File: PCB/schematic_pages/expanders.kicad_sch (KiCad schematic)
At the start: 32 parts

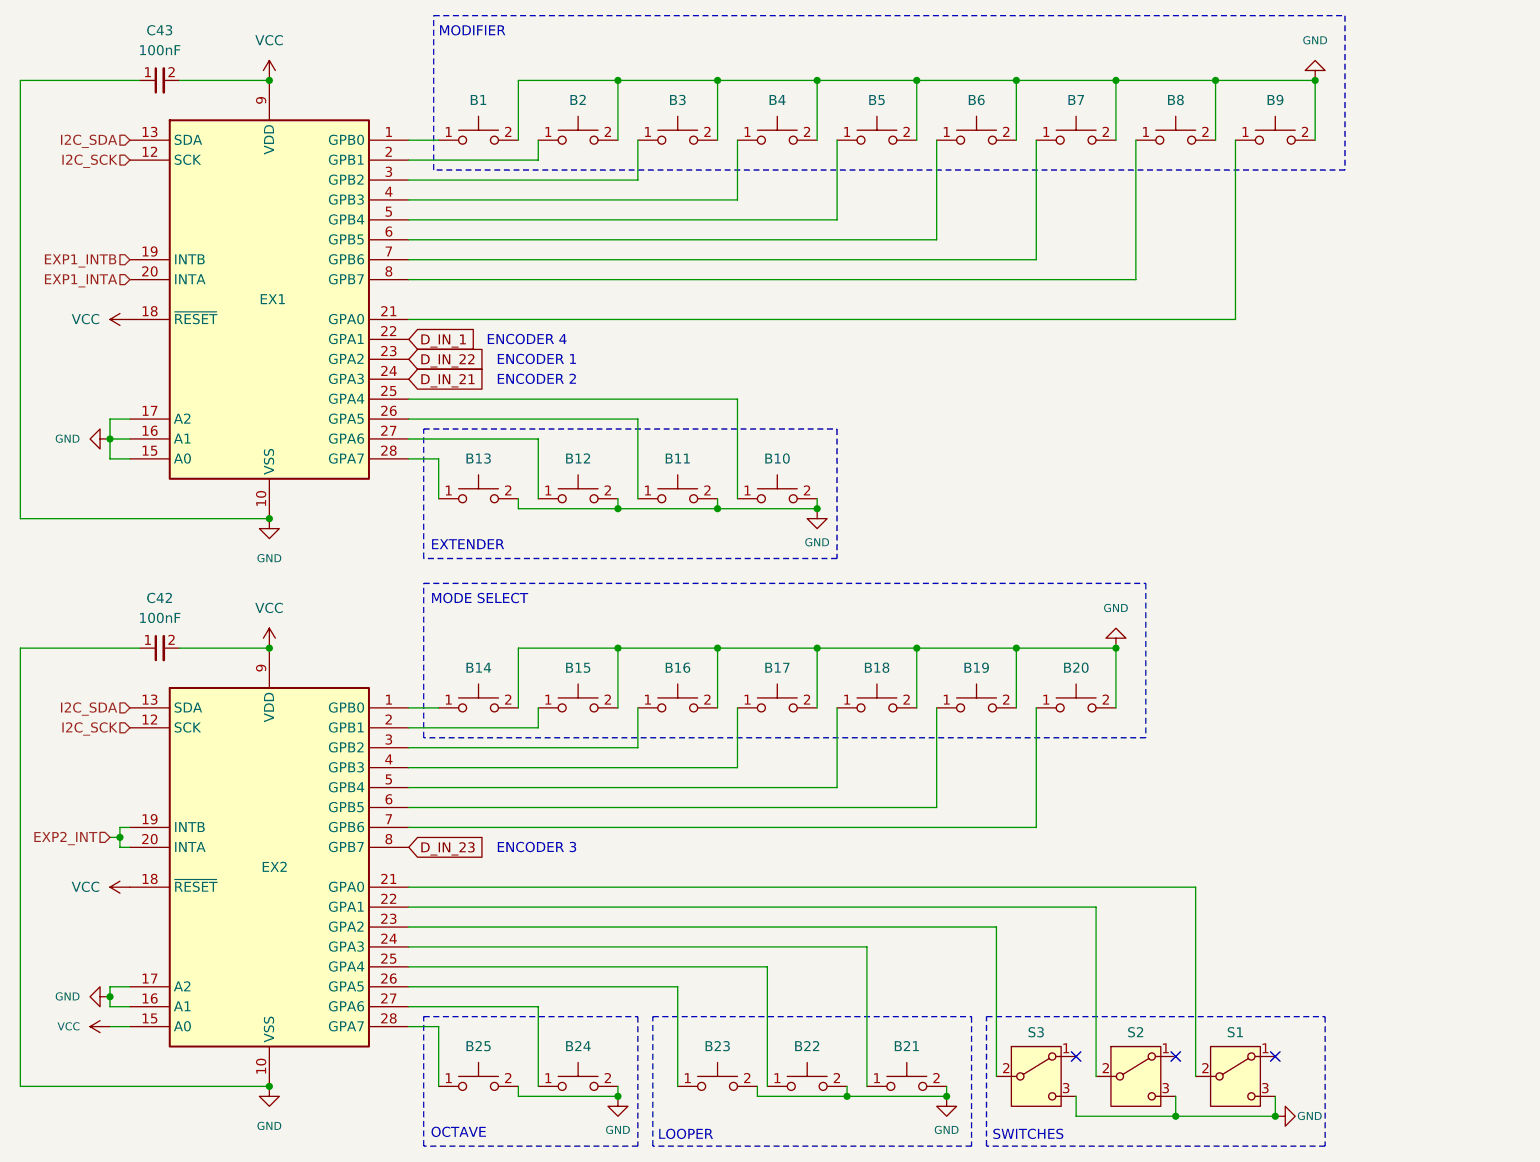
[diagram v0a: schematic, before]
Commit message: longahh day
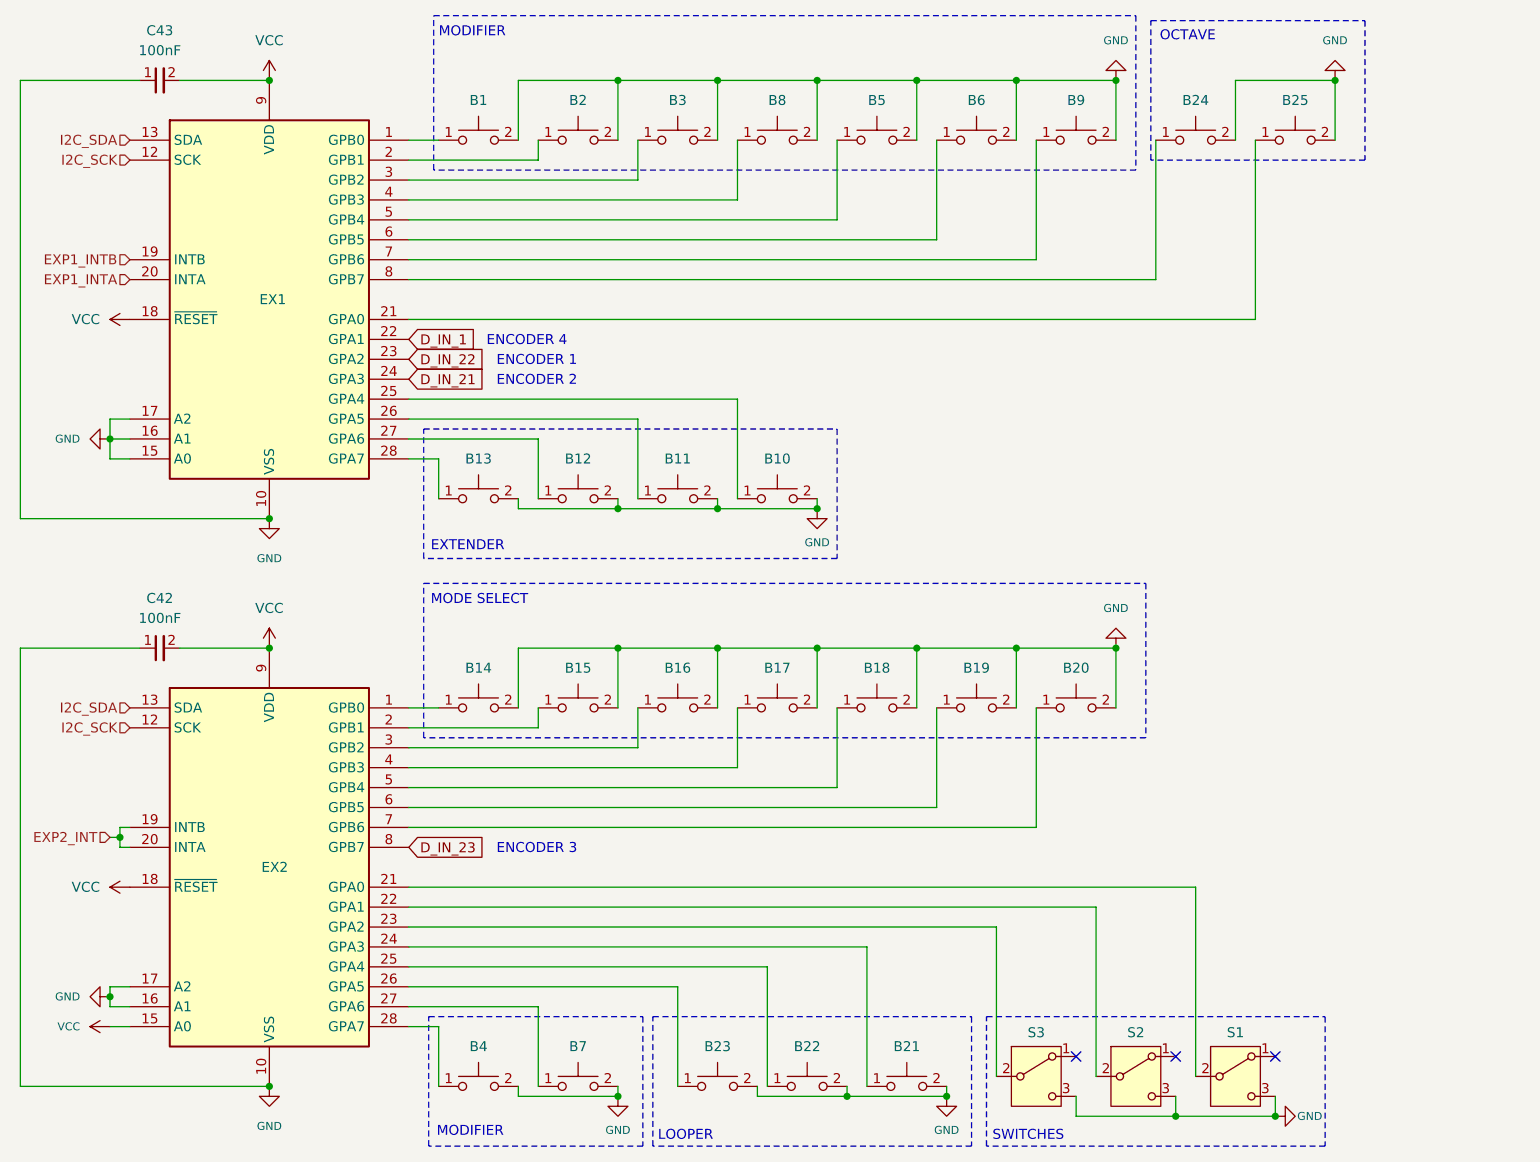
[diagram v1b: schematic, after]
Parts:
- renumbered B8 to B24, B9 to B25, B25 to B4, B24 to B7, B4 to B8, B7 to B9
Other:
- moved on the sheet: B24, B25
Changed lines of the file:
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@@
 	(paper "A4")
 	(rectangle
+		(start 105.41 143.51)
+		(end 132.715 160.02)
+		(stroke
+			(width 0)
+			(type dash)
+		)
+		(fill
+			(type none)
+		)
+	)
+	(rectangle
 		(start 176.53 143.51)
 		(end 219.71 160.02)
@@
 	(rectangle
 		(start 106.045 15.875)
-		(end 222.25 35.56)
+		(end 195.58 35.56)
 		(stroke
 			(width 0)
@@
 	)
 	(rectangle
-		(start 104.775 143.51)
-		(end 132.08 160.02)
+		(start 197.485 16.51)
+		(end 224.79 34.29)
 		(stroke
 			(width 0)
@@
 		)
 	)
+	(text "MODIFIER"
+		(exclude_from_sim no)
+		(at 106.426 158.242 0)
+		(effects
+			(font
+				(size 1.27 1.27)
+			)
+			(justify left)
+		)
+	)
 	(text "MODE SELECT"
 		(exclude_from_sim no)
@@
 	(text "OCTAVE"
 		(exclude_from_sim no)
-		(at 105.664 158.496 0)
+		(at 198.628 18.542 0)
 		(effects
 			(font
@@
 	)
 	(junction
+		(at 193.04 24.13)
+		(diameter 0)
+		(color 0 0 0 1)
+	)
+	(junction
 		(at 180.34 96.52)
 		(diameter 0)
@@
 	)
 	(junction
-		(at 218.44 24.13)
-		(diameter 0)
-		(color 0 0 0 1)
-	)
-	(junction
-		(at 193.04 24.13)
+		(at 220.98 24.13)
 		(diameter 0)
 		(color 0 0 0 1)
@@
 	)
 	(junction
-		(at 205.74 24.13)
-		(diameter 0)
-		(color 0 0 0 1)
-	)
-	(junction
 		(at 180.34 24.13)
 		(diameter 0)
@@
 	(wire
 		(pts
-			(xy 102.87 49.53) (xy 195.58 49.53)
+			(xy 102.87 49.53) (xy 198.12 49.53)
 		)
 		(stroke
@@
 	(wire
 		(pts
-			(xy 208.28 54.61) (xy 208.28 31.75)
+			(xy 210.82 54.61) (xy 210.82 31.75)
 		)
 		(stroke
@@
 	(wire
 		(pts
-			(xy 205.74 24.13) (xy 205.74 31.75)
+			(xy 208.28 24.13) (xy 208.28 31.75)
 		)
 		(stroke
@@
 	(wire
 		(pts
-			(xy 218.44 24.13) (xy 218.44 31.75)
+			(xy 220.98 24.13) (xy 220.98 31.75)
 		)
 		(stroke
@@
 	(wire
 		(pts
-			(xy 195.58 49.53) (xy 195.58 31.75)
+			(xy 198.12 49.53) (xy 198.12 31.75)
 		)
 		(stroke
@@
 	(wire
 		(pts
-			(xy 205.74 24.13) (xy 218.44 24.13)
+			(xy 208.28 24.13) (xy 220.98 24.13)
 		)
 		(stroke
@@
 	(wire
 		(pts
-			(xy 102.87 54.61) (xy 208.28 54.61)
+			(xy 102.87 54.61) (xy 210.82 54.61)
 		)
 		(stroke
@@
 	(wire
 		(pts
-			(xy 193.04 24.13) (xy 205.74 24.13)
-		)
-		(stroke
-			(width 0)
-			(type default)
-			(color 0 0 0 1)
-		)
-	)
-	(wire
-		(pts
 			(xy 102.87 36.83) (xy 132.08 36.83)
 		)
@@
 	(symbol
 		(lib_id "Symbols:GND")
-		(at 218.44 24.13 180)
+		(at 220.98 24.13 180)
 		(unit 1)
 		(exclude_from_sim no)
@@
 		(fields_autoplaced yes)
 		(property "Reference" "#PWR0106"
-			(at 218.44 24.13 0)
+			(at 220.98 24.13 0)
 			(effects
 				(font
@@
 		)
 		(property "Value" "GND"
-			(at 218.44 19.05 0)
+			(at 220.98 19.05 0)
 			(effects
 				(font
@@
 		)
 		(property "Footprint" ""
-			(at 218.44 24.13 0)
+			(at 220.98 24.13 0)
 			(effects
 				(font
@@
 		)
 		(property "Datasheet" ""
-			(at 218.44 24.13 0)
+			(at 220.98 24.13 0)
 			(effects
 				(font
@@
 		)
 		(property "Description" ""
-			(at 218.44 24.13 0)
+			(at 220.98 24.13 0)
 			(effects
 				(font
@@
 	)
 	(symbol
+		(lib_id "Symbols:GND")
+		(at 193.04 24.13 180)
+		(unit 1)
+		(exclude_from_sim no)
+		(in_bom yes)
+		(on_board yes)
+		(dnp no)
+		(fields_autoplaced yes)
+		(property "Reference" "#PWR0107"
+			(at 193.04 24.13 0)
+			(effects
+				(font
+					(size 1.27 1.27)
+				)
+				(hide yes)
+			)
+		)
+		(property "Value" "GND"
+			(at 193.04 19.05 0)
+			(effects
+				(font
+					(size 1.016 1.016)
+				)
+			)
+		)
+		(property "Footprint" ""
+			(at 193.04 24.13 0)
+			(effects
+				(font
+					(size 1.27 1.27)
+				)
+				(hide yes)
+			)
+		)
+		(property "Datasheet" ""
+			(at 193.04 24.13 0)
+			(effects
+				(font
+					(size 1.27 1.27)
+				)
+				(hide yes)
+			)
+		)
+		(property "Description" ""
+			(at 193.04 24.13 0)
+			(effects
+				(font
+					(size 1.27 1.27)
+				)
+				(hide yes)
+			)
+		)
+		(pin ""
+		)
+		(instances
+			(project "Harmora"
+				(path "/de43e009-b04c-42c1-b131-cdc664039a0d/8f5845f6-f6f8-4f8f-ac6e-d033b6efee1b"
+					(reference "#PWR0107")
+					(unit 1)
+				)
+			)
+		)
+	)
+	(symbol
 		(lib_id "power:VCC")
 		(at 67.31 127 90)
@@
 		(dnp no)
 		(fields_autoplaced yes)
-		(property "Reference" "B25"
+		(property "Reference" "B4"
 			(at 111.76 147.32 0)
 			(effects
@@
 			(project "Harmora"
 				(path "/de43e009-b04c-42c1-b131-cdc664039a0d/8f5845f6-f6f8-4f8f-ac6e-d033b6efee1b"
-					(reference "B25")
+					(reference "B4")
 					(unit 1)
 				)
@@
 		(dnp no)
 		(fields_autoplaced yes)
-		(property "Reference" "B7"
+		(property "Reference" "B9"
 			(at 187.96 26.67 0)
 			(effects
@@
 			(project "MCU_328p"
 				(path "/de43e009-b04c-42c1-b131-cdc664039a0d/8f5845f6-f6f8-4f8f-ac6e-d033b6efee1b"
-					(reference "B7")
+					(reference "B9")
 					(unit 1)
 				)
@@
 	(symbol
 		(lib_id "Symbols:Push_Switch")
-		(at 213.36 31.75 0)
+		(at 215.9 31.75 0)
 		(unit 1)
 		(exclude_from_sim no)
@@
 		(dnp no)
 		(fields_autoplaced yes)
-		(property "Reference" "B9"
-			(at 213.36 26.67 0)
+		(property "Reference" "B25"
+			(at 215.9 26.67 0)
 			(effects
 				(font
@@
 		)
 		(property "Value" "~"
-			(at 213.36 31.75 0)
+			(at 215.9 31.75 0)
 			(effects
 				(font
@@
 		)
 		(property "Footprint" "Footprints:Mechanical Switch"
-			(at 213.36 31.75 0)
+			(at 215.9 31.75 0)
 			(effects
 				(font
@@
 		)
 		(property "Datasheet" ""
-			(at 213.36 31.75 0)
+			(at 215.9 31.75 0)
 			(effects
 				(font
@@
 		)
 		(property "Description" ""
-			(at 213.36 31.75 0)
+			(at 215.9 31.75 0)
 			(effects
 				(font
@@
 			(project "MCU_328p"
 				(path "/de43e009-b04c-42c1-b131-cdc664039a0d/8f5845f6-f6f8-4f8f-ac6e-d033b6efee1b"
-					(reference "B9")
+					(reference "B25")
 					(unit 1)
 				)
@@
 		(dnp no)
 		(fields_autoplaced yes)
-		(property "Reference" "B4"
+		(property "Reference" "B8"
 			(at 149.86 26.67 0)
 			(effects
@@
 			(project "MCU_328p"
 				(path "/de43e009-b04c-42c1-b131-cdc664039a0d/8f5845f6-f6f8-4f8f-ac6e-d033b6efee1b"
-					(reference "B4")
+					(reference "B8")
 					(unit 1)
 				)
@@
 		(dnp no)
 		(fields_autoplaced yes)
-		(property "Reference" "B24"
+		(property "Reference" "B7"
 			(at 124.46 147.32 0)
 			(effects
@@
 			(project "Harmora"
 				(path "/de43e009-b04c-42c1-b131-cdc664039a0d/8f5845f6-f6f8-4f8f-ac6e-d033b6efee1b"
-					(reference "B24")
+					(reference "B7")
 					(unit 1)
 				)
@@
 	(symbol
 		(lib_id "Symbols:Push_Switch")
-		(at 200.66 31.75 0)
+		(at 203.2 31.75 0)
 		(unit 1)
 		(exclude_from_sim no)
@@
 		(dnp no)
 		(fields_autoplaced yes)
-		(property "Reference" "B8"
-			(at 200.66 26.67 0)
+		(property "Reference" "B24"
+			(at 203.2 26.67 0)
 			(effects
 				(font
@@
 		)
 		(property "Value" "~"
-			(at 200.66 31.75 0)
+			(at 203.2 31.75 0)
 			(effects
 				(font
@@
 		)
 		(property "Footprint" "Footprints:Mechanical Switch"
-			(at 200.66 31.75 0)
+			(at 203.2 31.75 0)
 			(effects
 				(font
@@
 		)
 		(property "Datasheet" ""
-			(at 200.66 31.75 0)
+			(at 203.2 31.75 0)
 			(effects
 				(font
@@
 		)
 		(property "Description" ""
-			(at 200.66 31.75 0)
+			(at 203.2 31.75 0)
 			(effects
 				(font
@@
 			(project "MCU_328p"
 				(path "/de43e009-b04c-42c1-b131-cdc664039a0d/8f5845f6-f6f8-4f8f-ac6e-d033b6efee1b"
-					(reference "B8")
+					(reference "B24")
 					(unit 1)
 				)

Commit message: pc is being
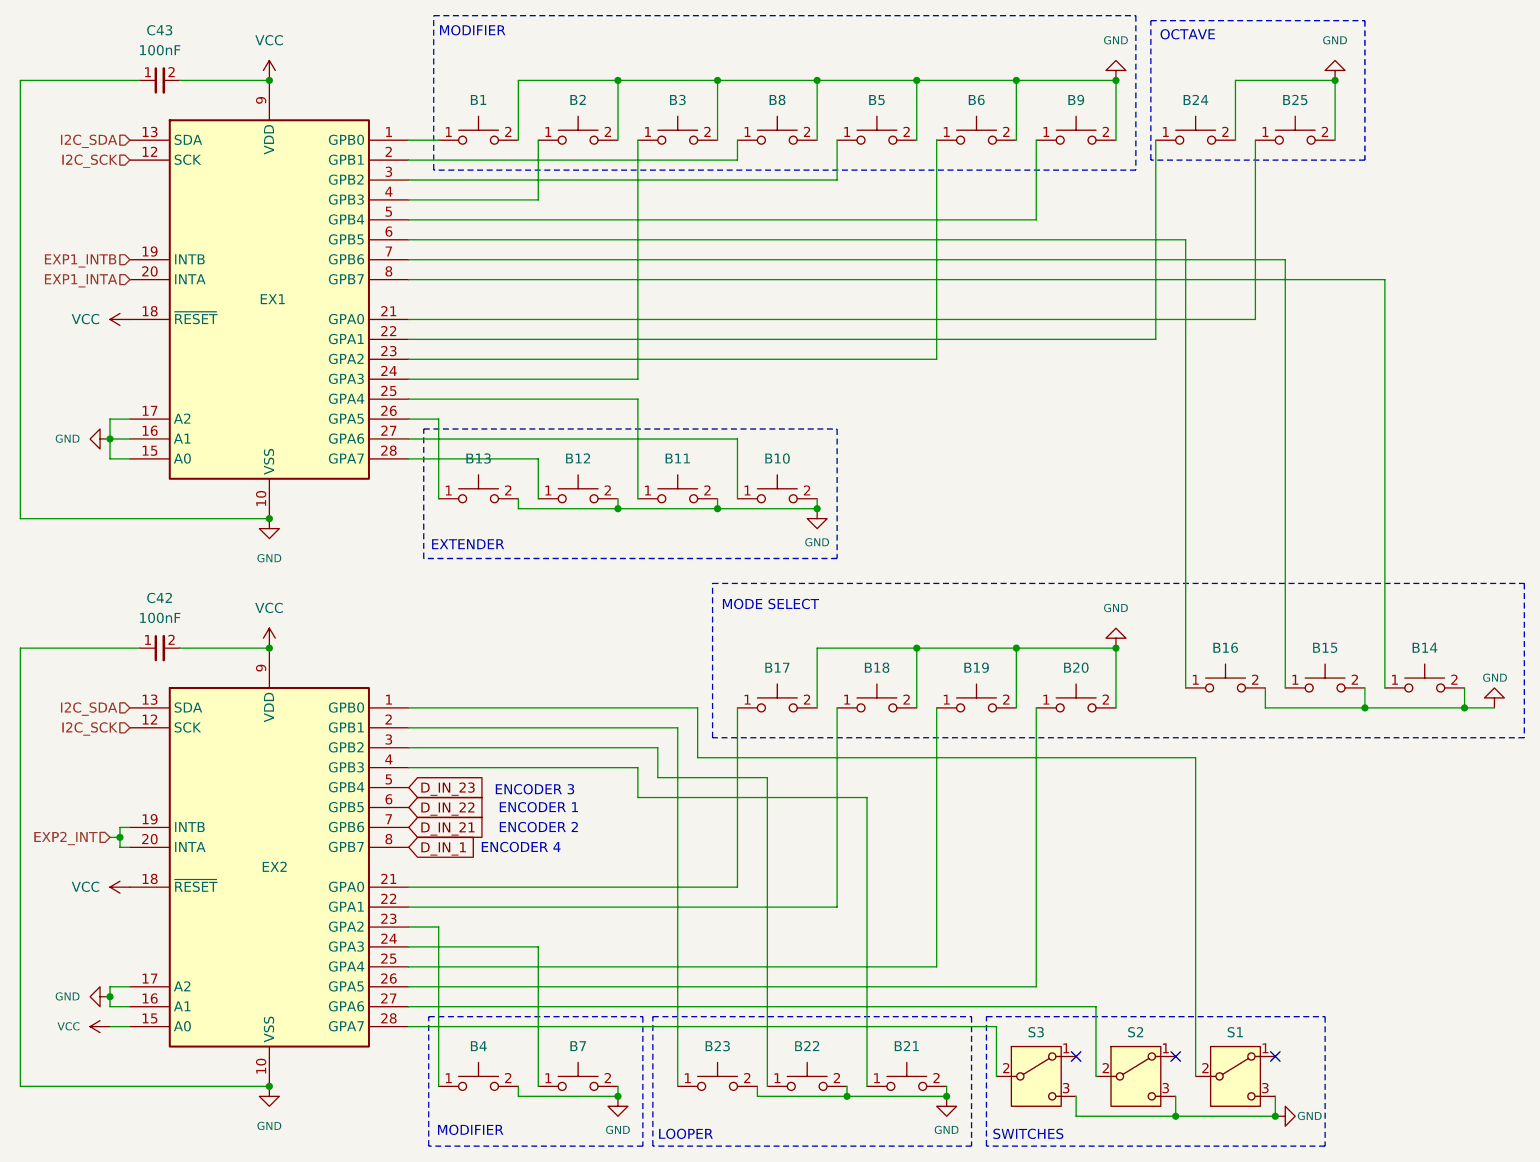
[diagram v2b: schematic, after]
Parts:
- renumbered B16 to B14, B14 to B16
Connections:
- net D_IN_1: now also EX2.8 (GPB7); no longer EX1.22 (GPA1)
- net D_IN_21: now also EX2.7 (GPB6); no longer EX1.24 (GPA3)
- net D_IN_22: now also EX2.6 (GPB5); no longer EX1.23 (GPA2)
- net D_IN_23: now also EX2.5 (GPB4); no longer EX2.8 (GPB7)
- net at B16.1: now also EX1.6 (GPB5); no longer EX2.1 (GPB0)
- net at B6.1: now also EX1.23 (GPA2); no longer EX1.6 (GPB5)
- net at EX2.2 (GPB1): now also B23.1; no longer B15.1
- net at S1.2: now also EX2.1 (GPB0); no longer EX2.21 (GPA0)
- net at EX2.22 (GPA1): now also B18.1; no longer S2.2
- net at EX2.23 (GPA2): now also B4.1; no longer S3.2
- net at EX2.24 (GPA3): now also B7.1; no longer B21.1
- net at EX2.25 (GPA4): now also B19.1; no longer B22.1
- net at EX2.26 (GPA5): now also B20.1; no longer B23.1
- net at EX2.27 (GPA6): now also S2.2; no longer B7.1
- net at EX2.28 (GPA7): now also S3.2; no longer B4.1
- net at EX2.3 (GPB2): now also B22.1; no longer B14.1
- net at B17.1: now also EX2.21 (GPA0); no longer EX2.4 (GPB3)
- net at EX1.7 (GPB6): now also B15.1; no longer B9.1
- net at B10.1: now also EX1.27 (GPA6); no longer EX1.25 (GPA4)
- net at EX1.2 (GPB1): now also B8.1; no longer B2.1
- net at B11.1: now also EX1.25 (GPA4); no longer EX1.26 (GPA5)
- net at B12.1: now also EX1.28 (GPA7); no longer EX1.27 (GPA6)
- net at B13.1: now also EX1.26 (GPA5); no longer EX1.28 (GPA7)
- net at B3.1: now also EX1.24 (GPA3); no longer EX1.3 (GPB2)
- net at EX1.4 (GPB3): now also B2.1; no longer B8.1
- net at EX1.5 (GPB4): now also B9.1; no longer B5.1
- net at EX1.8 (GPB7): now also B14.1; no longer B24.1
- new net: B21.1, EX2.4 (GPB3)
- new net: B24.1, EX1.22 (GPA1)
- new net: B5.1, EX1.3 (GPB2)
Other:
- moved on the sheet: B14, B15, B16
